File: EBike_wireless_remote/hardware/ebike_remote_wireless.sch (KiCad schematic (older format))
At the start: 6 parts

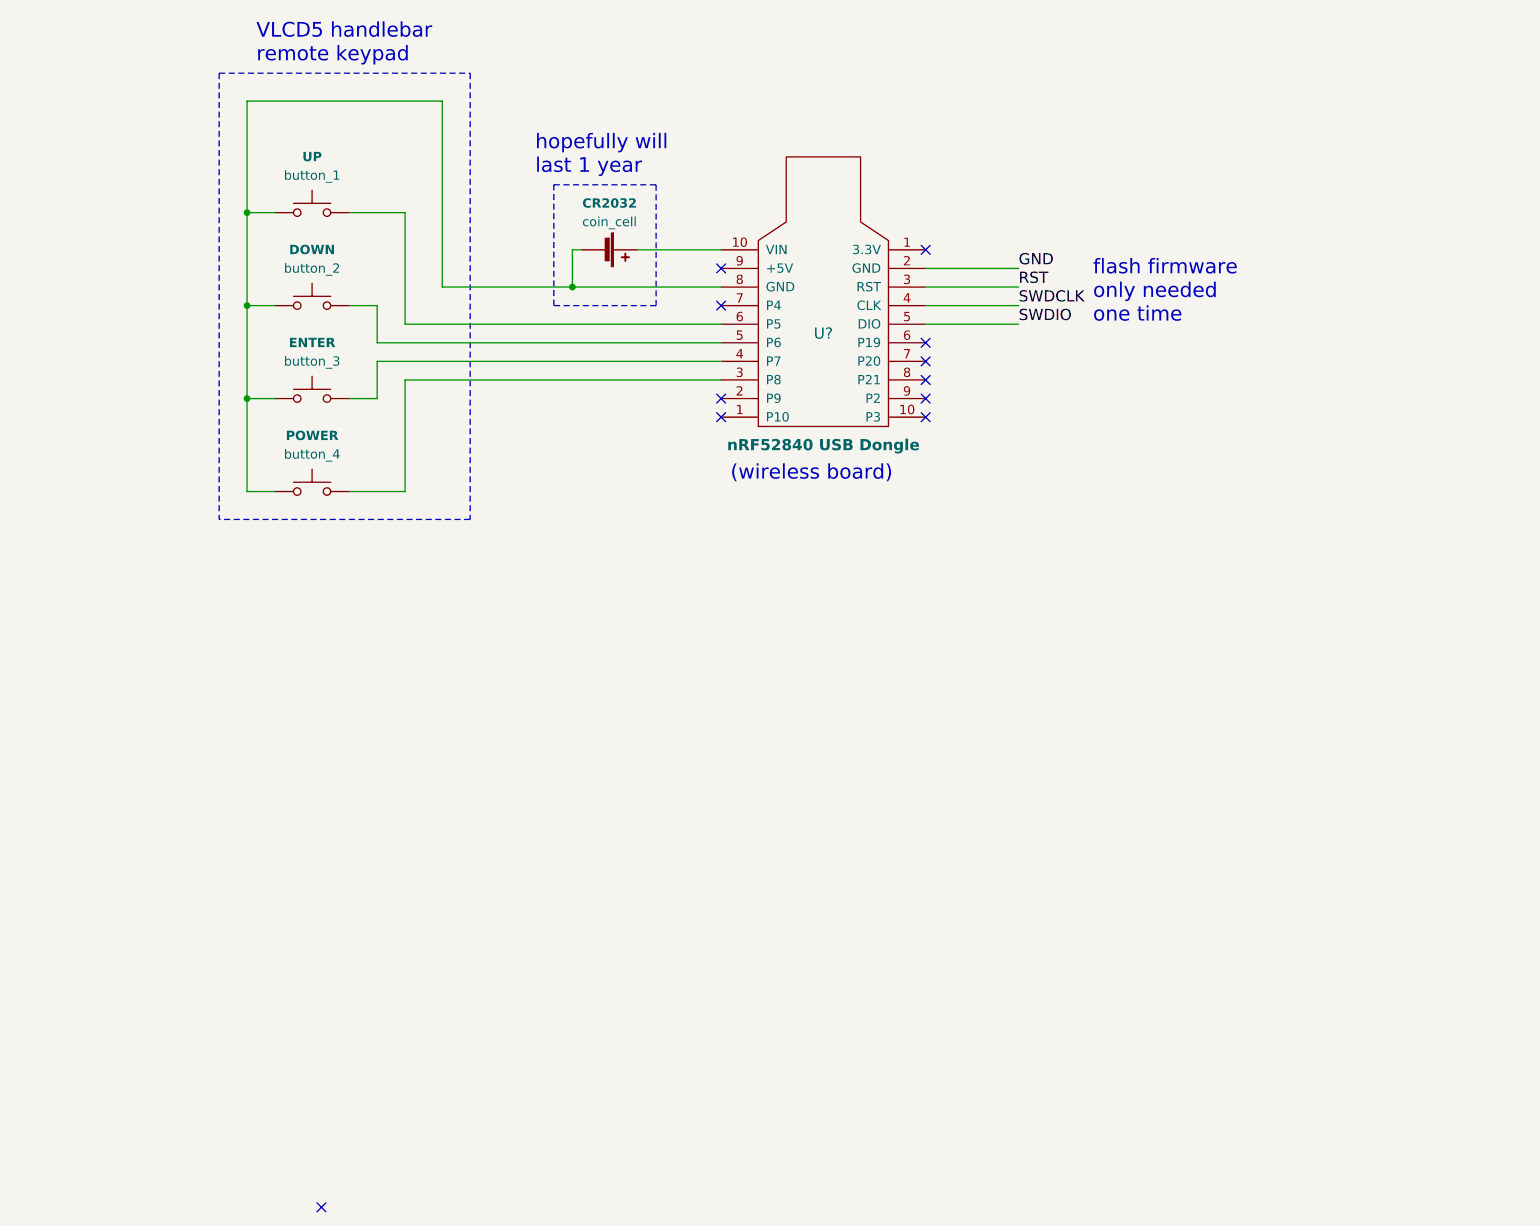
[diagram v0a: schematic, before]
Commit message: Updated schematics
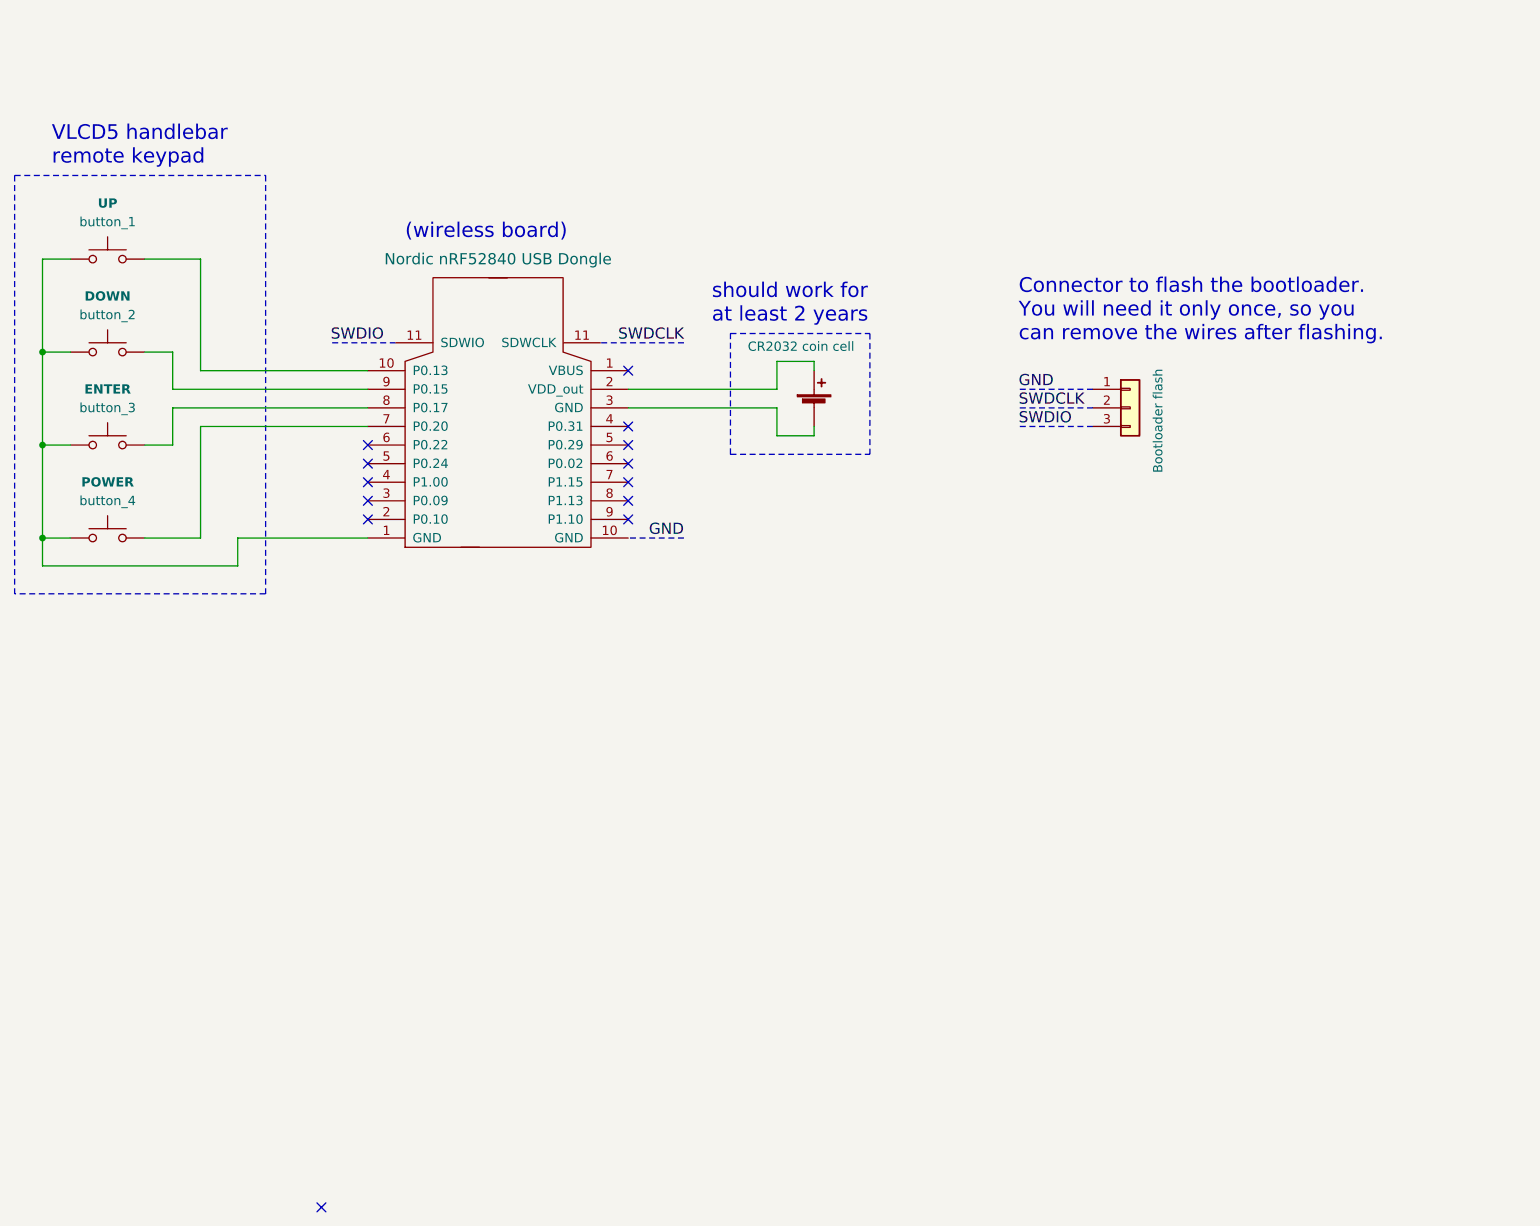
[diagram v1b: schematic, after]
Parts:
- removed U?: nRF52840 USB Dongle, symbol Dongle:nRF52840
- removed coin_cell: CR2032, symbol Device:Battery_Cell
- added J?: Bootloader flash, symbol Connector_Generic:Conn_01x03
- added U?: Nordic nRF52840 USB Dongle, symbol Wireless_eBike:Nordic_nRF52840_USB_Dongle
- added coincell: CR2032 coin cell, symbol Device:Battery_Cell
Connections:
- net at button_4.2: now also U?.7 (P1.15)
- net at button_3.2: now also U?.8 (P1.13)
- net at button_2.2: now also U?.9 (P1.10)
- net at button_1.2: now also U?.10 (P0.13)
- net at button_1.1, button_2.1, button_3.1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: now also U?.1 (VBUS)
- new net: U?.2 (VDD_out), coincell.1 (+)
- new net: U?.3 (P0.09), coincell.2 (-)
- no-connect marks 11 -> 13
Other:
- note added: "Connector to flash the bootloader.\nYou will need it only once, so you\ncan remove the wires after flashing."
- note added: "should work for\nat least 2 years"
- note removed: "flash firmware\nonly needed\none time"
- note removed: "hopefully will\nlast 1 year"
- moved on the sheet: button_1, button_2, button_3, button_4
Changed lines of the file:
@@
 Comment4 ""
 $EndDescr
-NoConn ~ 7050 2950
-Text Label 7550 3050 0    60   ~ 0
-GND
-Text Label 7550 3150 0    60   ~ 0
-RST
-Text Label 7550 3250 0    60   ~ 0
-SWDCLK
-Text Label 7550 3350 0    60   ~ 0
-SWDIO
 NoConn ~ 3800 8100
-$Comp
-L Dongle:nRF52840 U?
-U 1 1 5EEB15B7
-P 6500 3450
-F 0 "U?" H 6500 3500 60  0000 C CNN
-F 1 "nRF52840 USB Dongle" H 6500 2900 60  0000 C CNB
-F 2 "" H 6500 3450 60  0000 C CNN
-F 3 "" H 6500 3450 60  0000 C CNN
-	1    6500 3450
-	1    0    0    -1
-$EndComp
-Wire Wire Line
-	7050 3050 7550 3050
-Wire Wire Line
-	7050 3150 7550 3150
-Wire Wire Line
-	7050 3250 7550 3250
-Wire Wire Line
-	7050 3350 7550 3350
-NoConn ~ 7050 3450
-NoConn ~ 7050 3550
-NoConn ~ 7050 3650
-NoConn ~ 7050 3750
-NoConn ~ 7050 3850
-NoConn ~ 5950 3850
-NoConn ~ 5950 3750
-NoConn ~ 5950 3050
-NoConn ~ 5950 3250
-$Comp
-L Device:Battery_Cell coin_cell
-U 1 1 5F4A3162
-P 5300 2950
-F 0 "coin_cell" V 5150 3000 50  0000 C CNN
-F 1 "CR2032" V 5050 3000 50  0000 C CNB
-F 2 "" V 5300 3010 50  0001 C CNN
-F 3 "~" V 5300 3010 50  0001 C CNN
-	1    5300 2950
-	0    1    1    0
-$EndComp
 $Comp
 L Switch:SW_Push button_1
 U 1 1 5F4A3714
-P 3750 2750
-F 0 "button_1" H 3750 2950 50  0000 C CNN
-F 1 "UP" H 3750 3050 50  0000 C CNB
-F 2 "" H 3750 2950 50  0001 C CNN
-F 3 "~" H 3750 2950 50  0001 C CNN
-	1    3750 2750
-	1    0    0    -1
-$EndComp
+P 2650 3000
+F 0 "button_1" H 2650 3200 50  0000 C CNN
+F 1 "UP" H 2650 3300 50  0000 C CNB
+F 2 "" H 2650 3200 50  0001 C CNN
+F 3 "~" H 2650 3200 50  0001 C CNN
+	1    2650 3000
+	1    0    0    -1
+$EndComp
+Wire Wire Line
+	2300 3000 2450 3000
+Wire Wire Line
+	3150 3900 4050 3900
+Connection ~ 2300 4000
+Wire Wire Line
+	2300 4000 2450 4000
+$Comp
+L Switch:SW_Push button_3
+U 1 1 5F4A4B3B
+P 2650 4000
+F 0 "button_3" H 2650 4200 50  0000 C CNN
+F 1 "ENTER" H 2650 4300 50  0000 C CNB
+F 2 "" H 2650 4200 50  0001 C CNN
+F 3 "~" H 2650 4200 50  0001 C CNN
+	1    2650 4000
+	1    0    0    -1
+$EndComp
+Connection ~ 2300 3500
+Wire Wire Line
+	2300 4000 2300 3500
+Wire Wire Line
+	2300 3500 2300 3000
+Wire Wire Line
+	2300 3500 2450 3500
+$Comp
+L Switch:SW_Push button_2
+U 1 1 5F4A3F33
+P 2650 3500
+F 0 "button_2" H 2650 3700 50  0000 C CNN
+F 1 "DOWN" H 2650 3800 50  0000 C CNB
+F 2 "" H 2650 3700 50  0001 C CNN
+F 3 "~" H 2650 3700 50  0001 C CNN
+	1    2650 3500
+	1    0    0    -1
+$EndComp
+Wire Wire Line
+	2850 4000 3000 4000
+Wire Wire Line
+	3000 4000 3000 3800
+Wire Wire Line
+	3000 3800 4050 3800
+Wire Wire Line
+	4050 3700 3000 3700
+Wire Wire Line
+	3000 3700 3000 3500
+Wire Wire Line
+	3000 3500 2850 3500
+Wire Wire Line
+	2850 3000 3150 3000
+Wire Wire Line
+	3150 3000 3150 3600
+Wire Wire Line
+	3150 3600 4050 3600
+Wire Notes Line
+	2150 2550 3500 2550
+Wire Notes Line
+	3500 2550 3500 4800
+Wire Notes Line
+	3500 4800 2150 4800
+Wire Notes Line
+	2150 2550 2150 4800
+Text Notes 4250 2900 0    79   ~ 0
+(wireless board)
+Text Notes 7550 3450 0    79   ~ 0
+Connector to flash the bootloader.\nYou will need it only once, so you\ncan remove the wires after flashing.
+Text Notes 2350 2500 0    79   ~ 0
+VLCD5 handlebar\nremote keypad
+$Comp
+L Wireless_eBike:Nordic_nRF52840_USB_Dongle U?
+U 1 1 600AD575
+P 4750 3950
+F 0 "U?" H 4750 4987 60  0001 C CNN
+F 1 "Nordic nRF52840 USB Dongle" H 4750 4900 60  0000 C CNN
+F 2 "" H 4600 3800 60  0000 C CNN
+F 3 "" H 4600 3800 60  0000 C CNN
+	1    4750 3950
+	1    0    0    -1
+$EndComp
+Wire Notes Line
+	6000 4050 6000 3400
+Wire Notes Line
+	6000 3400 6750 3400
+Text Notes 5900 3350 0    79   ~ 0
+should work for\nat least 2 years
+$Comp
+L Device:Battery_Cell coincell
+U 1 1 600B4826
+P 6450 3800
+F 0 "coincell" V 6300 3850 50  0001 C CNN
+F 1 "CR2032 coin cell" H 6380 4130 50  0000 C CNN
+F 2 "" V 6450 3860 50  0001 C CNN
+F 3 "~" V 6450 3860 50  0001 C CNN
+	1    6450 3800
+	1    0    0    -1
+$EndComp
+Wire Wire Line
+	2850 4500 3150 4500
+Wire Wire Line
+	2300 4500 2300 4000
+Wire Wire Line
+	3150 4500 3150 3900
+Wire Wire Line
+	2450 4500 2300 4500
 $Comp
 L Switch:SW_Push button_4
 U 1 1 5F4A4B45
-P 3750 4250
-F 0 "button_4" H 3750 4450 50  0000 C CNN
-F 1 "POWER" H 3750 4550 50  0000 C CNB
-F 2 "" H 3750 4450 50  0001 C CNN
-F 3 "~" H 3750 4450 50  0001 C CNN
-	1    3750 4250
-	1    0    0    -1
-$EndComp
-Wire Wire Line
-	5500 2950 5950 2950
-Wire Wire Line
-	5150 3150 5150 2950
-Wire Wire Line
-	5150 2950 5200 2950
-Wire Wire Line
-	3550 4250 3400 4250
-Wire Wire Line
-	3400 2750 3550 2750
-Wire Wire Line
-	4250 4250 4250 3650
-Wire Wire Line
-	4250 3650 5950 3650
-Connection ~ 3400 3750
-Wire Wire Line
-	3400 4250 3400 3750
-Wire Wire Line
-	3400 3750 3550 3750
-$Comp
-L Switch:SW_Push button_3
-U 1 1 5F4A4B3B
-P 3750 3750
-F 0 "button_3" H 3750 3950 50  0000 C CNN
-F 1 "ENTER" H 3750 4050 50  0000 C CNB
-F 2 "" H 3750 3950 50  0001 C CNN
-F 3 "~" H 3750 3950 50  0001 C CNN
-	1    3750 3750
-	1    0    0    -1
-$EndComp
-Connection ~ 3400 3250
-Wire Wire Line
-	3400 3750 3400 3250
-Wire Wire Line
-	3400 3250 3400 2750
-Wire Wire Line
-	3400 3250 3550 3250
-$Comp
-L Switch:SW_Push button_2
-U 1 1 5F4A3F33
-P 3750 3250
-F 0 "button_2" H 3750 3450 50  0000 C CNN
-F 1 "DOWN" H 3750 3550 50  0000 C CNB
-F 2 "" H 3750 3450 50  0001 C CNN
-F 3 "~" H 3750 3450 50  0001 C CNN
-	1    3750 3250
-	1    0    0    -1
-$EndComp
-Wire Wire Line
-	3950 3750 4100 3750
-Wire Wire Line
-	4100 3750 4100 3550
-Wire Wire Line
-	4100 3550 5950 3550
-Wire Wire Line
-	5950 3450 4100 3450
-Wire Wire Line
-	4100 3450 4100 3250
-Wire Wire Line
-	4100 3250 3950 3250
-Wire Wire Line
-	3950 4250 4250 4250
-Wire Wire Line
-	3950 2750 4250 2750
-Wire Wire Line
-	4250 2750 4250 3350
-Wire Wire Line
-	3400 2750 3400 2150
-Wire Wire Line
-	3400 2150 4450 2150
-Wire Wire Line
-	4450 2150 4450 3150
-Wire Wire Line
-	4450 3150 5150 3150
-Connection ~ 3400 2750
-Connection ~ 5150 3150
-Wire Wire Line
-	5150 3150 5950 3150
-Wire Wire Line
-	4250 3350 5950 3350
-Wire Notes Line
-	3250 2000 4600 2000
-Wire Notes Line
-	4600 2000 4600 4400
-Wire Notes Line
-	4600 4400 3250 4400
-Wire Notes Line
-	3250 2000 3250 4400
-Wire Notes Line
-	5050 3250 5050 2600
-Wire Notes Line
-	5050 2600 5600 2600
-Wire Notes Line
-	5600 2600 5600 3250
-Wire Notes Line
-	5600 3250 5050 3250
-Text Notes 6000 4200 0    79   ~ 0
-(wireless board)
-Text Notes 7950 3350 0    79   ~ 0
-flash firmware\nonly needed\none time
-Text Notes 4950 2550 0    79   ~ 0
-hopefully will\nlast 1 year
-Text Notes 3450 1950 0    79   ~ 0
-VLCD5 handlebar\nremote keypad
+P 2650 4500
+F 0 "button_4" H 2650 4700 50  0000 C CNN
+F 1 "POWER" H 2650 4800 50  0000 C CNB
+F 2 "" H 2650 4700 50  0001 C CNN
+F 3 "~" H 2650 4700 50  0001 C CNN
+	1    2650 4500
+	1    0    0    -1
+$EndComp
+Wire Wire Line
+	2300 4500 2300 4650
+Wire Wire Line
+	2300 4650 3350 4650
+Wire Wire Line
+	3350 4650 3350 4500
+Wire Wire Line
+	3350 4500 4050 4500
+Connection ~ 2300 4500
+Wire Notes Line
+	6750 3400 6750 4050
+Wire Notes Line
+	6000 4050 6750 4050
+NoConn ~ 4050 4000
+NoConn ~ 4050 4100
+NoConn ~ 4050 4200
+NoConn ~ 4050 4300
+NoConn ~ 4050 4400
+NoConn ~ 5450 4400
+NoConn ~ 5450 4300
+NoConn ~ 5450 4200
+NoConn ~ 5450 4100
+NoConn ~ 5450 4000
+NoConn ~ 5450 3900
+Text Label 7550 3700 0    60   ~ 0
+GND
+Text Label 7550 3900 0    60   ~ 0
+SWDIO
+Text Label 7550 3800 0    60   ~ 0
+SWDCLK
+Text Label 5750 3450 2    60   ~ 0
+SWDCLK
+Text Label 5750 4500 2    60   ~ 0
+GND
+Text Label 3850 3450 0    60   ~ 0
+SWDIO
+Wire Notes Line style solid rgb(255, 114, 0)
+	4200 3450 3850 3450
+Wire Notes Line style solid rgb(255, 114, 0)
+	5750 3450 5300 3450
+Wire Notes Line style solid rgb(255, 114, 0)
+	5750 4500 5450 4500
+Wire Notes Line style solid rgb(255, 114, 0)
+	7950 3700 7550 3700
+Wire Notes Line style solid rgb(255, 114, 0)
+	7950 3800 7550 3800
+Wire Notes Line style solid rgb(255, 114, 0)
+	7950 3900 7550 3900
+Wire Wire Line
+	5450 3800 6250 3800
+Wire Wire Line
+	6250 3700 6250 3550
+Wire Wire Line
+	6250 3550 6450 3550
+Wire Wire Line
+	6450 3550 6450 3600
+Wire Wire Line
+	5450 3700 6250 3700
+Wire Wire Line
+	6250 3800 6250 3950
+Wire Wire Line
+	6250 3950 6450 3950
+Wire Wire Line
+	6450 3950 6450 3900
+$Comp
+L Connector_Generic:Conn_01x03 J?
+U 1 1 600C2D4C
+P 8150 3800
+F 0 "J?" H 8230 3842 50  0001 L CNN
+F 1 "Bootloader flash" V 8300 3450 50  0000 L CNN
+F 2 "" H 8150 3800 50  0001 C CNN
+F 3 "~" H 8150 3800 50  0001 C CNN
+	1    8150 3800
+	1    0    0    -1
+$EndComp
+NoConn ~ 5450 3600
 $EndSCHEMATC
